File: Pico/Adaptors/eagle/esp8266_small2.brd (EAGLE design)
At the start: 28.7 x 15.4 mm, 3 parts, among them U2 MCP1703T-3302E/CB

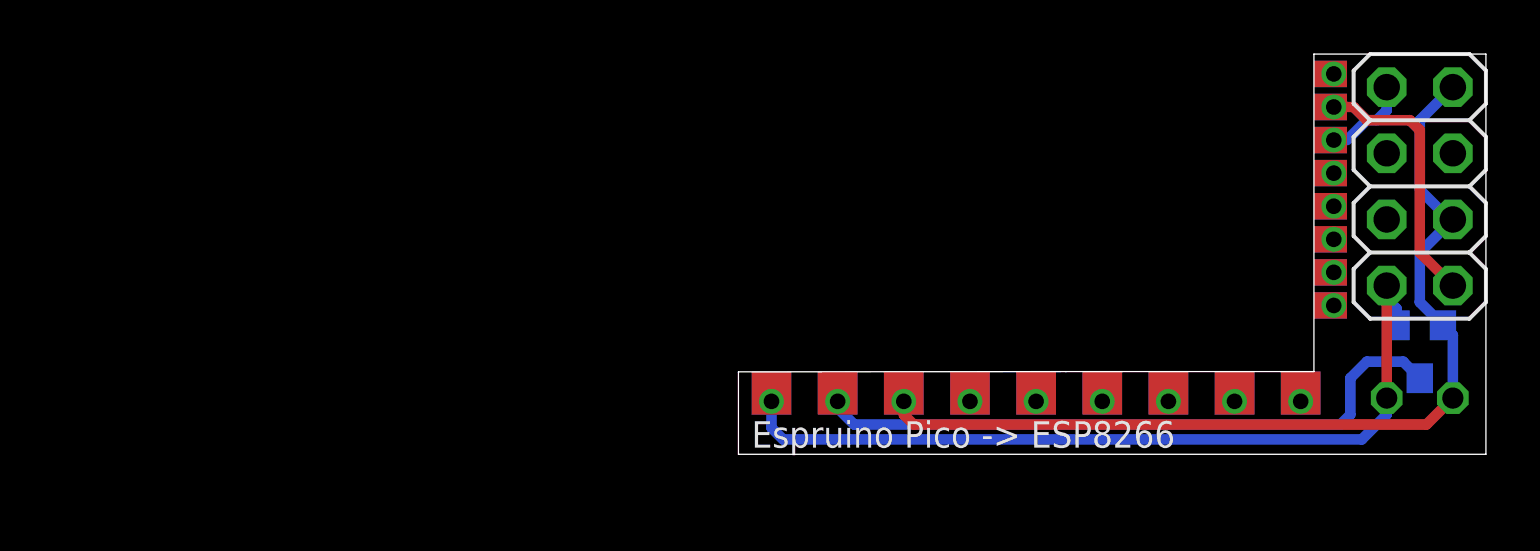
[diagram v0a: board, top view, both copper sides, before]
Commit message: more tweaks and options
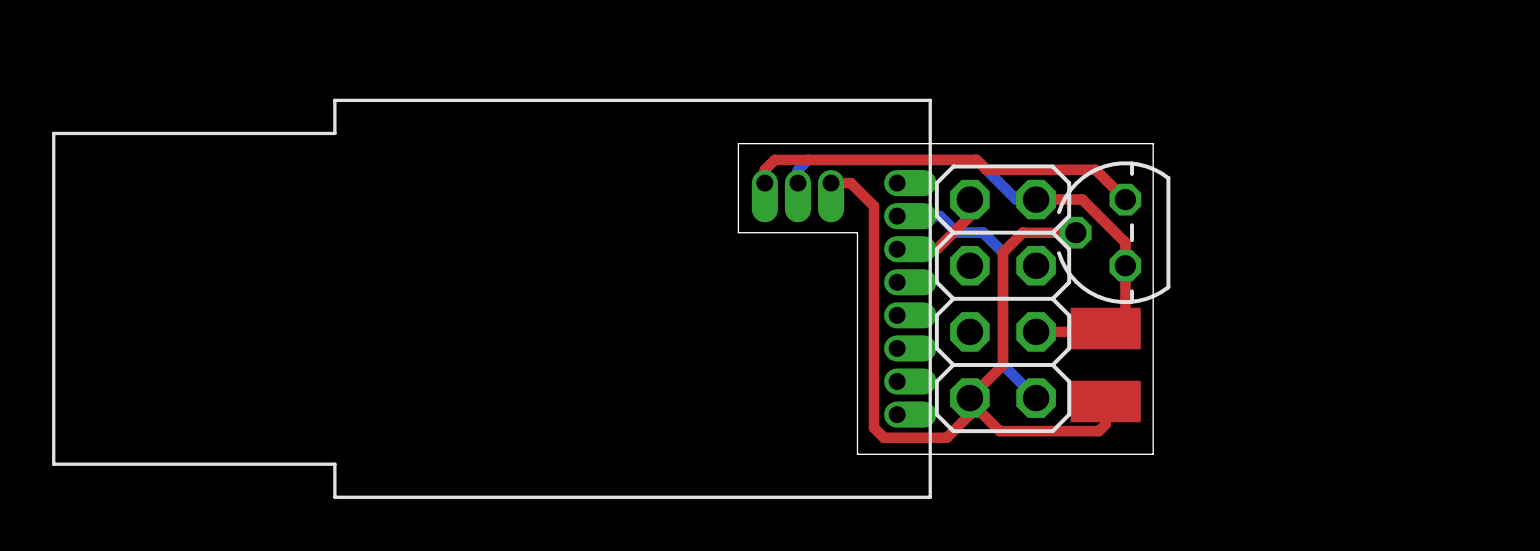
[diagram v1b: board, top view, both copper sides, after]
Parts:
- removed U2: MCP1703T-3302E/CB, xc6206:SOT23
- added IC2: 78L 3.3v, linear:TO92
- added U$1: ESPRUINO_PICO_0.05, espruino_pico:ESPRUINO_PICO_0.05
- C1: value (none) -> 22uF; device rcl:C025-050X050 -> rcl:C1210
- moved ESP8266 16.6 mm to (10.2, 5.97)
- moved C1 12.1 mm to (14.1, 3.43), flipped to the top, turned to 270 degrees
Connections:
- removed net 5V: U2.3
- removed net VSS: C1.2, ESP8266.7, U2.1
- new net GND: C1.2, ESP8266.7, IC2.2, U$1.GND_2
- new net N$1: IC2.3, U$1.5V_2
- net ESP_RX: now also U$1.A2
- net ESP_TX: now also U$1.A3
- net VCC: now also IC2.1, U$1.3.3V_2; no longer U2.2
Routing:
- net VSS: track 31.9 -> 0.00 mm, vias 1 -> 0
- net GND: track 0.00 -> 31.4 mm
- net 5V: track 24.9 -> 0.00 mm, vias 1 -> 0
- net VCC: track 36.8 -> 21.0 mm, vias 1 -> 0
- net N$1: track 0.00 -> 15.1 mm
- net ESP_RX: track 2.89 -> 3.96 mm
- net ESP_TX: track 10.2 -> 10.8 mm
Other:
- board size 28.7 x 15.4 mm -> 15.9 x 11.9 mm
- board text added: "Espruino ESP8266"
- board text removed: "Espruino Pico -> ESP8266"
